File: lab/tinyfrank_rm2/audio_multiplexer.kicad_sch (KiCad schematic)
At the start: 4 parts, among them U2 74HC4052D

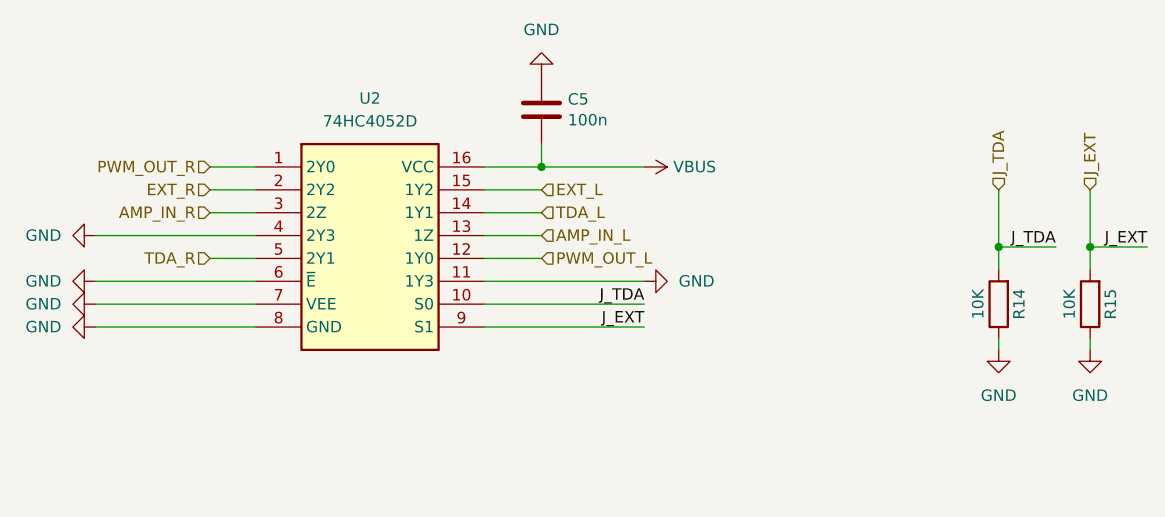
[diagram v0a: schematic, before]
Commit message: FRANK M1 + TinyFRANK RM2 WIP
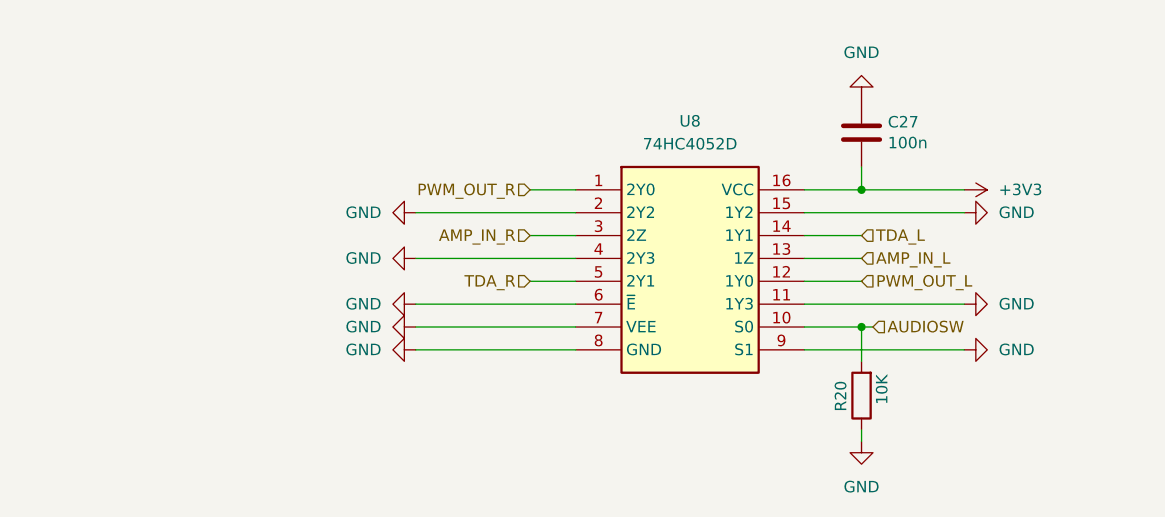
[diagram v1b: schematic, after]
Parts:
- removed C5: 100n, FRANK:Capacitor (0603, S), symbol Device:C
- removed R14, R15: 10K, FRANK:Resistor (0603, S), symbol Device:R
- removed U2: 74HC4052D, FRANK:SOP-16, symbol FRANK:74HC4052D
- added C27: 100n, FRANK:Capacitor (0805), symbol Device:C
- added R20: 10K, FRANK:Resistor (0805), symbol Device:R
- added U8: 74HC4052D, FRANK:74HC4052D653, symbol FRANK:74HC4052D
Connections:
- net AMP_IN_L: now also U8.13 (1Z)
- net AMP_IN_R: now also U8.3 (2Z)
- net GND: now also C27.1, R20.1, U8.11 (1Y3), U8.15 (1Y2), U8.2 (2Y2), U8.4 (2Y3), U8.6 (~{E}), U8.7 (VEE), U8.8 (GND), U8.9 (S1)
- net PWM_OUT_L: now also U8.12 (1Y0)
- net PWM_OUT_R: now also U8.1 (2Y0)
- net TDA_L: now also U8.14 (1Y1)
- net TDA_R: now also U8.5 (2Y1)
- new net +3V3: C27.2, U8.16 (VCC)
- new net AUDIOSW: R20.2, U8.10 (S0)
